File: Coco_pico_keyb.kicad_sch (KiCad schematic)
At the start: 3 parts, among them J1 Conn_01x16_Pin, J2 DE9_Plug_MountingHoles, U1 Pico

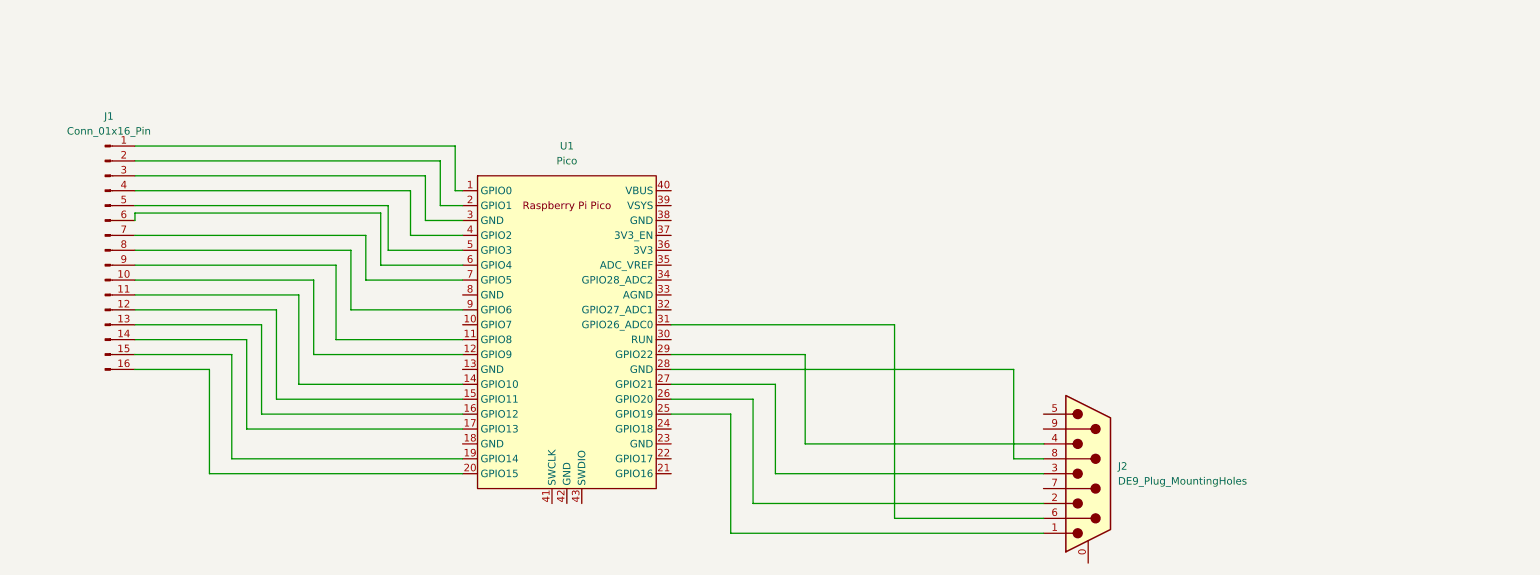
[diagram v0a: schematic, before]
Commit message: Latest version, first to be built.  100% tested now, works well
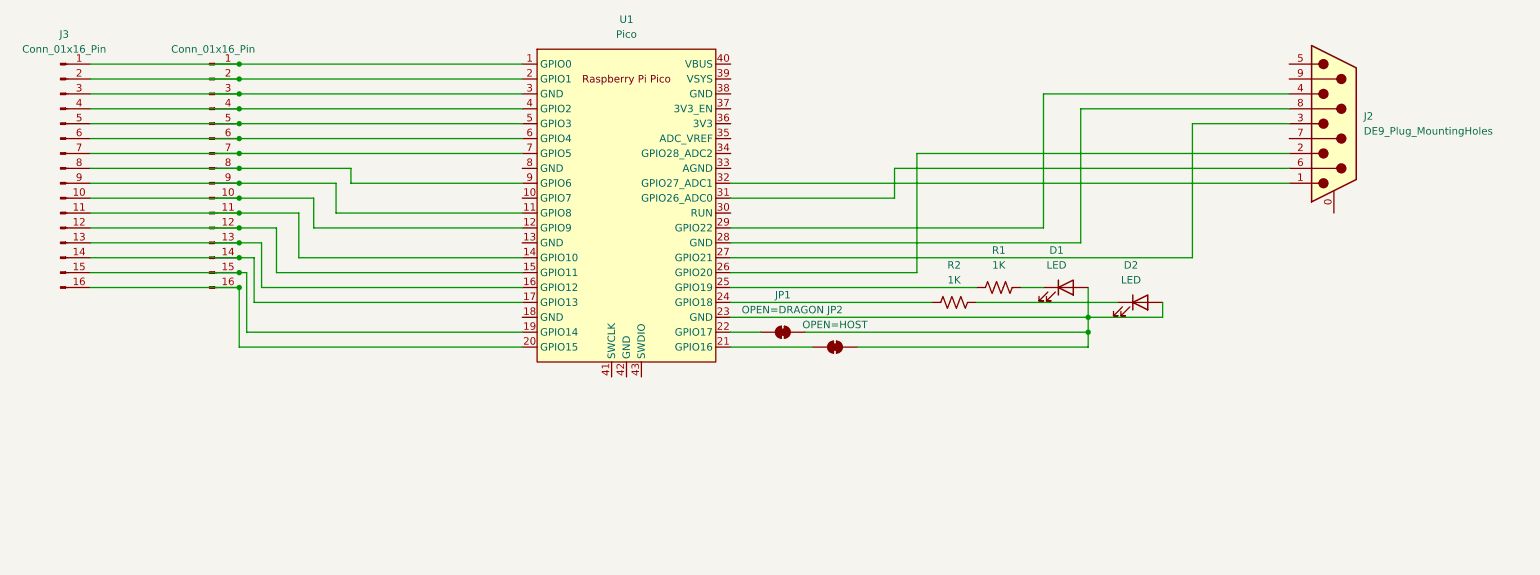
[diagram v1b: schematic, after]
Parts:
- added D1, D2: LED, LED_THT:LED_D3.0mm, symbol Device:LED
- added J3: Conn_01x16_Pin, Connector_PinHeader_2.54mm:PinHeader_1x16_P2.54mm_Vertical, symbol Connector:Conn_01x16_Pin
- added JP1: OPEN=DRAGON, Jumper:SolderJumper-2_P1.3mm_Open_RoundedPad1.0x1.5mm, symbol Jumper:SolderJumper_2_Bridged
- added JP2: OPEN=HOST, Jumper:SolderJumper-2_P1.3mm_Open_RoundedPad1.0x1.5mm, symbol Jumper:SolderJumper_2_Bridged
- added R1, R2: 1K, Resistor_THT:R_Axial_DIN0207_L6.3mm_D2.5mm_P7.62mm_Horizontal, symbol Device:R_US
- J1: footprint (none) -> Connector_PinHeader_2.54mm:PinHeader_1x16_P2.54mm_Vertical
- J2: footprint (none) -> Connector_Dsub:DSUB-9_Pins_Horizontal_P2.77x2.84mm_EdgePinOffset4.94mm_Housed_MountingHolesOffset4.94mm
- U1: footprint RPi_Pico:RPi_Pico_SMD_TH -> Module:RaspberryPi_Pico_Common_SMD
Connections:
- net at J2.1: now also U1.32 (GPIO27_ADC1); no longer U1.25 (GPIO19)
- net at J1.1 (Pin_1), U1.1 (GPIO0): now also J3.1 (Pin_1)
- net at J1.9 (Pin_9), U1.11 (GPIO8): now also J3.9 (Pin_9)
- net at J1.10 (Pin_10), U1.12 (GPIO9): now also J3.10 (Pin_10)
- net at J1.11 (Pin_11), U1.14 (GPIO10): now also J3.11 (Pin_11)
- net at J1.12 (Pin_12), U1.15 (GPIO11): now also J3.12 (Pin_12)
- net at J1.13 (Pin_13), U1.16 (GPIO12): now also J3.13 (Pin_13)
- net at J1.14 (Pin_14), U1.17 (GPIO13): now also J3.14 (Pin_14)
- net at J1.15 (Pin_15), U1.19 (GPIO14): now also J3.15 (Pin_15)
- net at J1.2 (Pin_2), U1.2 (GPIO1): now also J3.2 (Pin_2)
- net at J1.16 (Pin_16), U1.20 (GPIO15): now also J3.16 (Pin_16)
- net at U1.21 (GPIO16): now also JP2.1 (A)
- net at U1.22 (GPIO17): now also JP1.1 (A)
- net at U1.23 (GND): now also D1.2 (A), D2.2 (A), JP1.2 (B), JP2.2 (B)
- net at U1.24 (GPIO18): now also R2.1
- net at J1.3 (Pin_3), U1.3 (GND): now also J3.3 (Pin_3)
- net at J1.4 (Pin_4), U1.4 (GPIO2): now also J3.4 (Pin_4)
- net at J1.5 (Pin_5), U1.5 (GPIO3): now also J3.5 (Pin_5)
- net at J1.6 (Pin_6), U1.6 (GPIO4): now also J3.6 (Pin_6)
- net at J1.7 (Pin_7), U1.7 (GPIO5): now also J3.7 (Pin_7)
- net at J1.8 (Pin_8), U1.9 (GPIO6): now also J3.8 (Pin_8)
- new net: D1.1 (K), R1.2
- new net: D2.1 (K), R2.2
- new net: R1.1, U1.25 (GPIO19)
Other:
- moved on the sheet: J2, U1
